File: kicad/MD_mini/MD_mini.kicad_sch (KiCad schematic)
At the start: 52 parts, among them J1 Conn_01x02_Pin, J2 Conn_01x03_Pin, J3 Conn_01x02_Pin, J4 Conn_01x02_Pin, J6 Conn_02x03_Odd_Even, U1 IRS2003, U2 SCM3723ASA, U3 IRS2003, U4 ACS711xEXLT-15AB, U7 IRS2003, U8 IRS2003, U9 SCM3723ASA

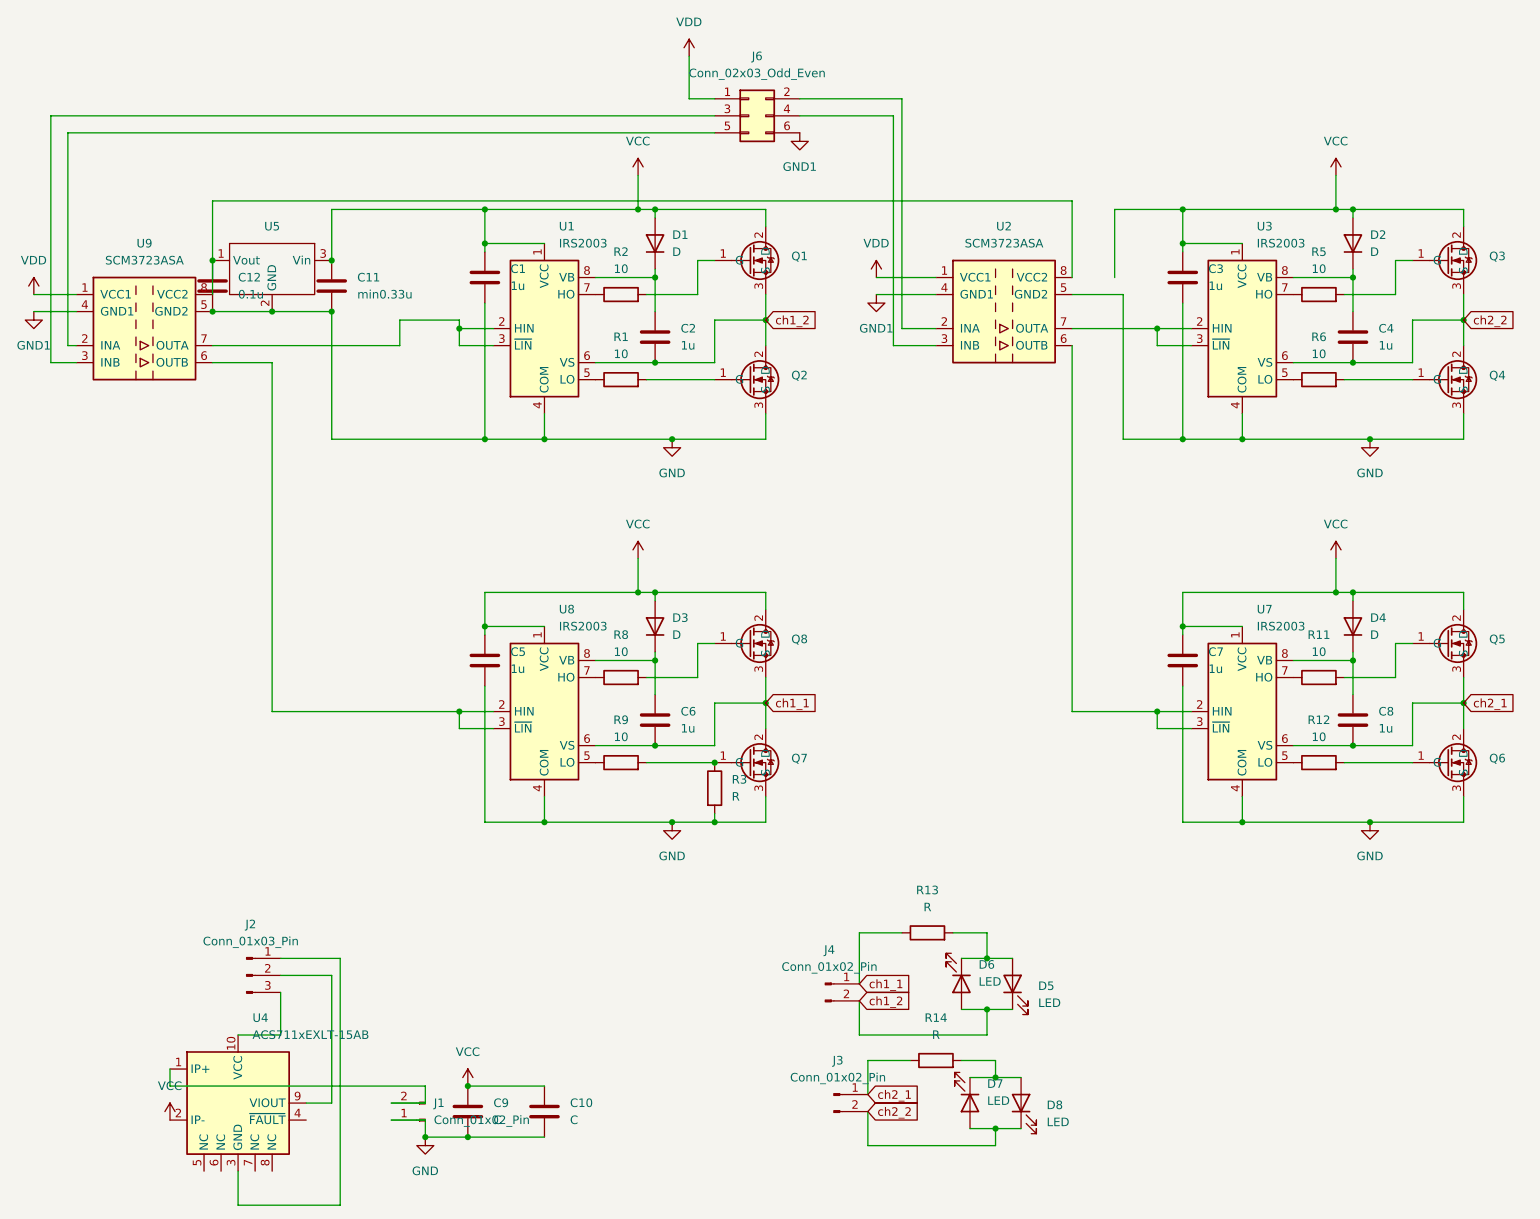
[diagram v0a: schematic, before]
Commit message: a
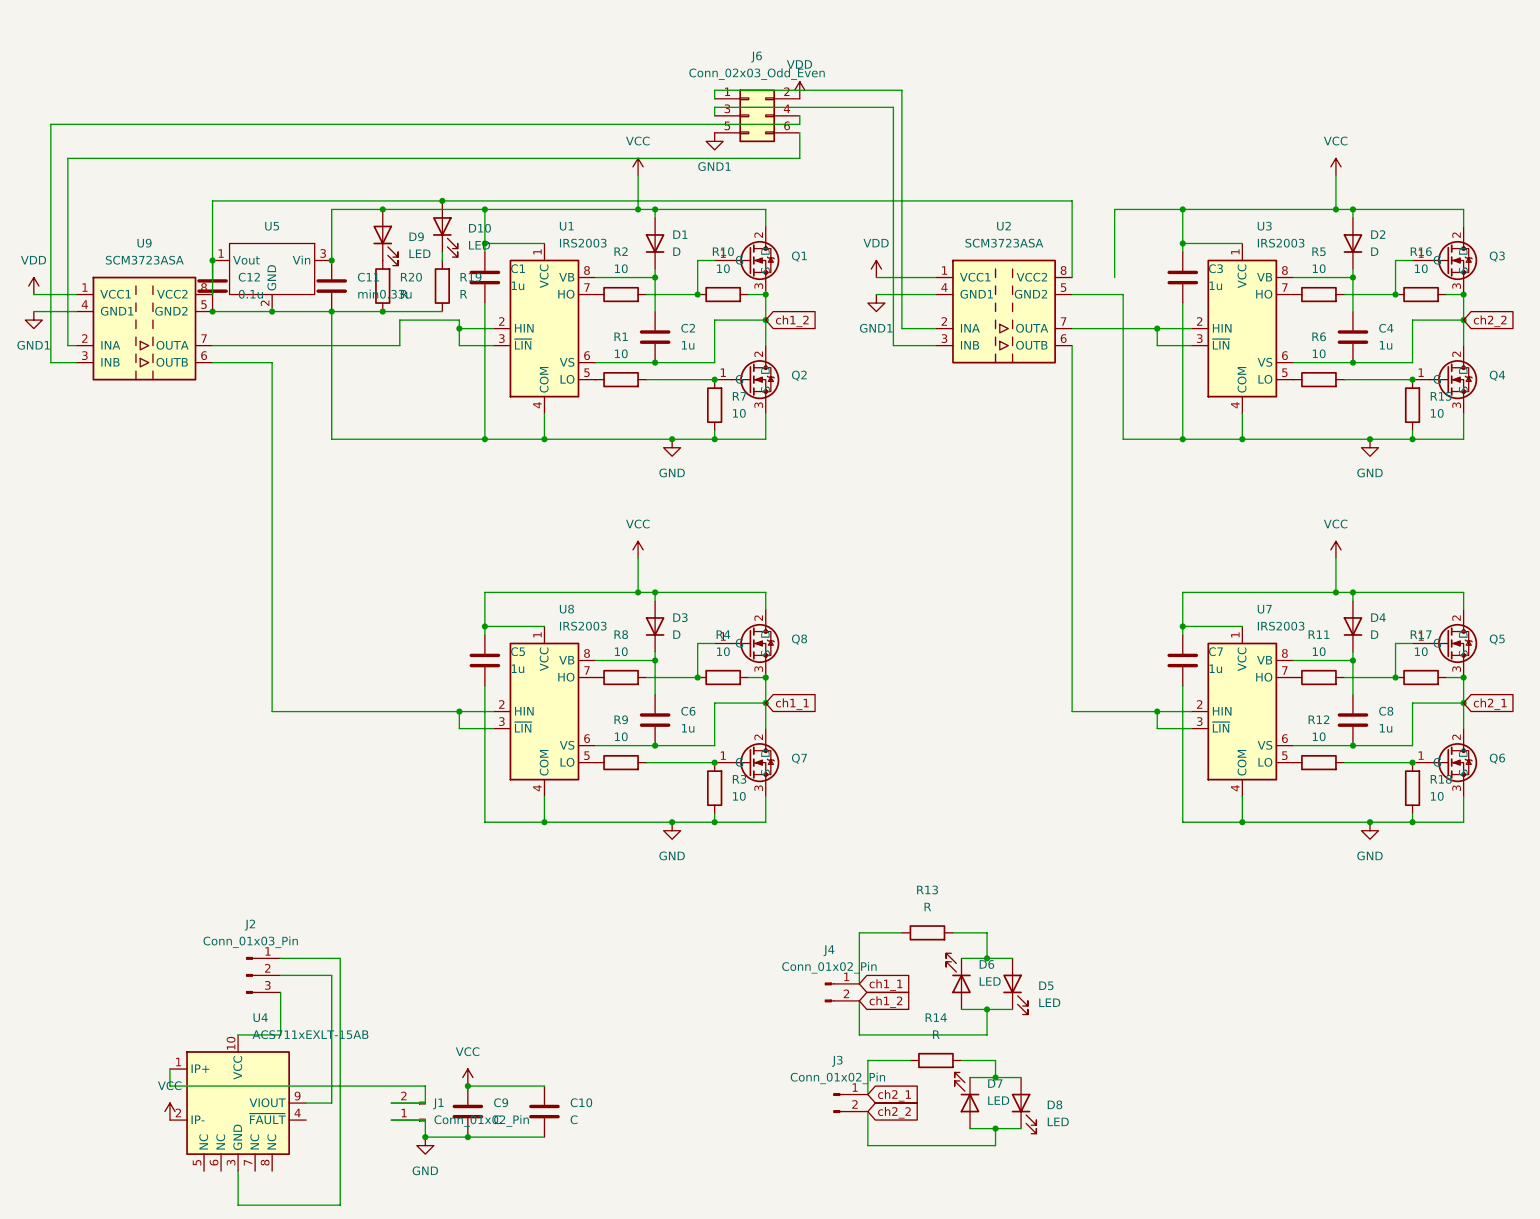
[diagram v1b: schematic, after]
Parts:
- added D10, D9: LED, LED_SMD:LED_0603_1608Metric_Pad1.05x0.95mm_HandSolder, symbol Device:LED
- added R10, R15, R16, R17, R18, R4, R7: 10, Resistor_SMD:R_0603_1608Metric_Pad0.98x0.95mm_HandSolder, symbol Device:R
- added R19, R20: R, Resistor_SMD:R_0603_1608Metric_Pad0.98x0.95mm_HandSolder, symbol Device:R
- R3: value R -> 10; footprint (none) -> Resistor_SMD:R_0603_1608Metric_Pad0.98x0.95mm_HandSolder
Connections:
- net GND: now also R3.1, R15.1, R18.1, R19.1, R20.1, R7.1; no longer R3.2
- net GND1: now also J6.5 (Pin_5); no longer J6.6 (Pin_6)
- net VCC: now also D9.2 (A)
- net VDD: now also J6.2 (Pin_2); no longer J6.1 (Pin_1)
- net ch1_1: now also R4.2
- net ch1_2: now also R10.2
- net ch2_1: now also R17.2
- net ch2_2: now also R16.2
- net at Q6.1 (G), R12.2: now also R18.2
- net at Q2.1 (G), R1.2: now also R7.2
- net at Q7.1 (G), R9.2: now also R3.2; no longer R3.1
- net at U9.2 (INA): now also J6.6 (Pin_6); no longer J6.5 (Pin_5)
- net at U9.3 (INB): now also J6.4 (Pin_4); no longer J6.3 (Pin_3)
- net at C12.1, U2.8 (VCC2), U5.1 (Vout)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: now also D10.2 (A)
- net at Q4.1 (G), R6.2: now also R15.2
- net at Q1.1 (G), R2.2: now also R10.1
- net at Q5.1 (G), R11.2: now also R17.1
- net at Q3.1 (G), R5.2: now also R16.1
- net at U2.2 (INA): now also J6.1 (Pin_1); no longer J6.2 (Pin_2)
- net at U2.3 (INB): now also J6.3 (Pin_3); no longer J6.4 (Pin_4)
- net at Q8.1 (G), R8.2: now also R4.1
- new net: D9.1 (K), R20.2
- new net: D10.1 (K), R19.2
